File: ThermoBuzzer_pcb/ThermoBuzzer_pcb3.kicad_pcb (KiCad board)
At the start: 2 copper layers, 61 x 59.7 mm, 10 parts, among them SW2 SW_Push

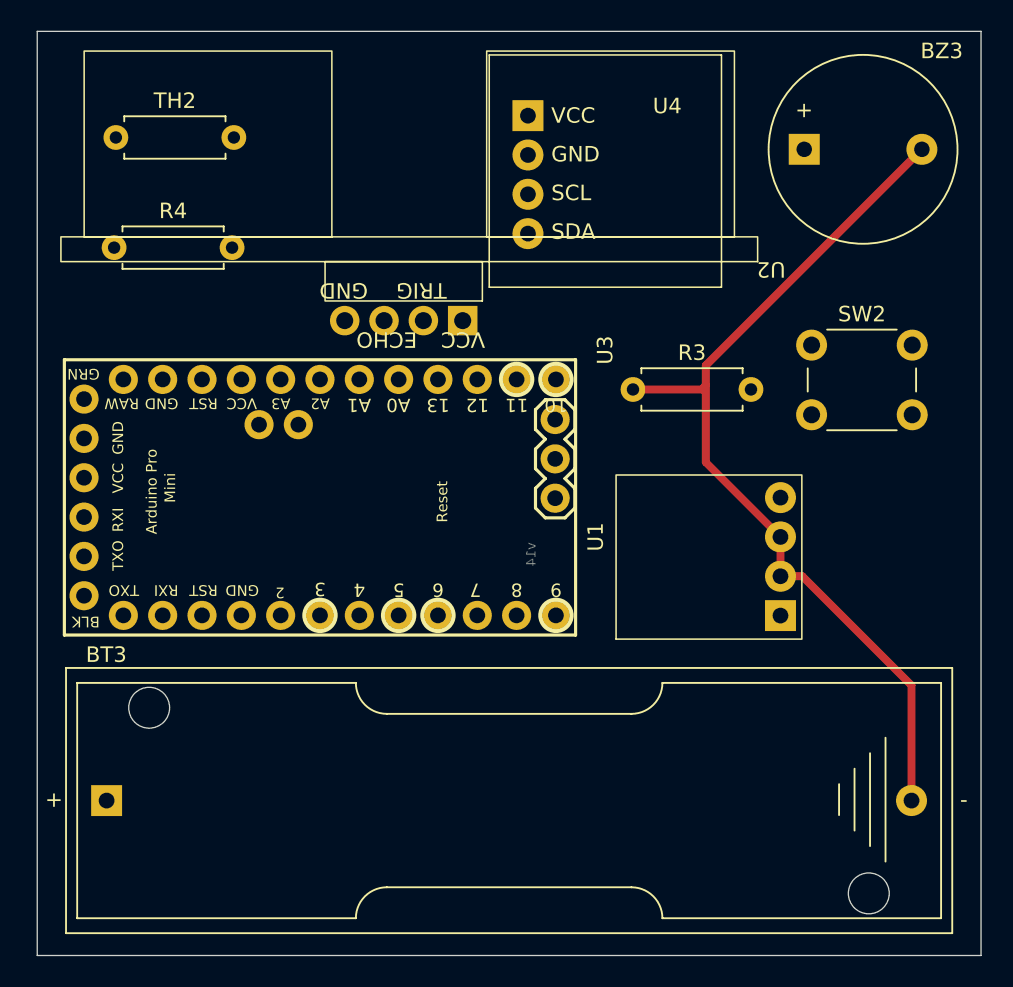
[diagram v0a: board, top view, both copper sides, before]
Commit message: 4.23
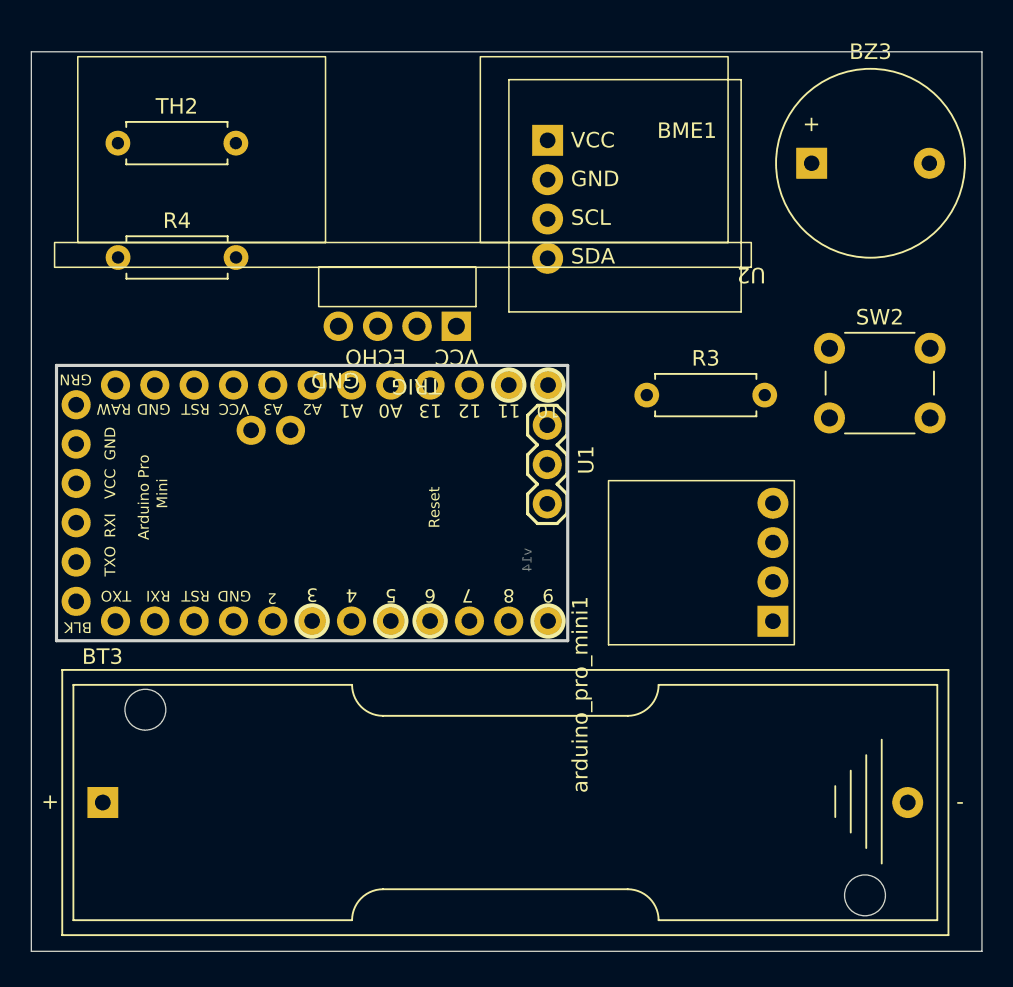
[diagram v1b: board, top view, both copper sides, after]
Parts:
- moved BME1 2.04 mm to (131.4, 79.7)
- moved SW2 1.17 mm to (145.2, 89.0)
- moved BZ3 1.02 mm to (144.0, 77.1)
- moved R3 0.96 mm to (133.3, 92.1)
- moved R4 0.68 mm to (99.2, 83.2)
- moved arduino_pro_mini1 0.63 mm to (127.1, 106.5)
- moved U1 0.61 mm to (133.9, 88.9)
- moved U2 0.55 mm to (140.1, 83.8)
- moved TH2 0.39 mm to (99.2, 75.8)
- moved BT3 0.28 mm to (98.2, 118.4)
- renumbered U4 to BME1, U3 to U1, U1 to arduino_pro_mini1
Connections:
- BME1 pad 2: Net-(U4-GND) -> GND
- R4 pad 2: Net-(U4-GND) -> GND
- arduino_pro_mini1 pad r2: Net-(U4-GND) -> unconnected-(arduino_pro_mini1-GND-Padr2)
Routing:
- net GND: track 59.0 -> 0.00 mm
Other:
- board size 61 x 59.7 mm -> 61.4 x 58.1 mm
